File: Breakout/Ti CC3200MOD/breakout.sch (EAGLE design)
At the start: 69 parts, among them Q1 16Mhz, U1 TPS63001DRCT, U11 XL, U12 TMP006, U2 MCP73871-2CCI/ML, U5 93LC46BT-I/OT

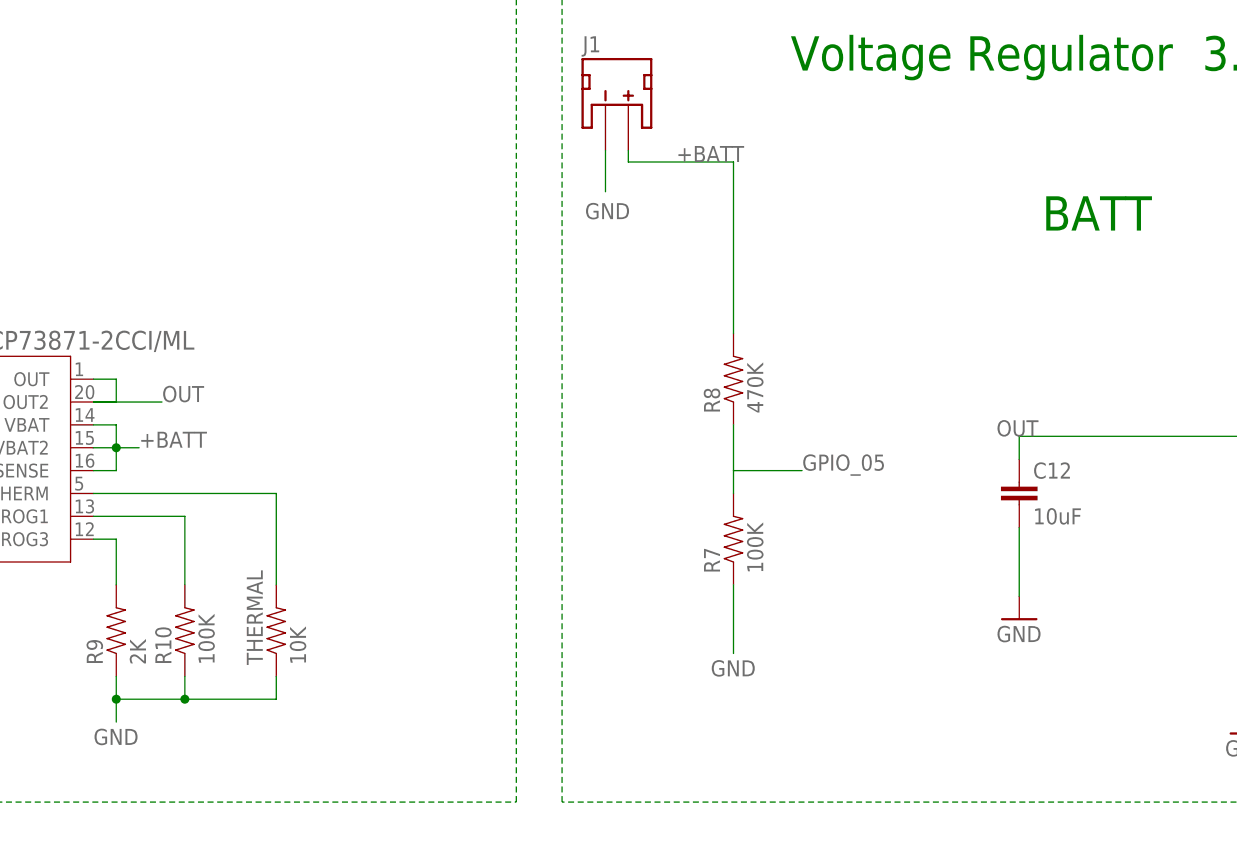
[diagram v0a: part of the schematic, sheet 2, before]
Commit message: Add Power Jumper
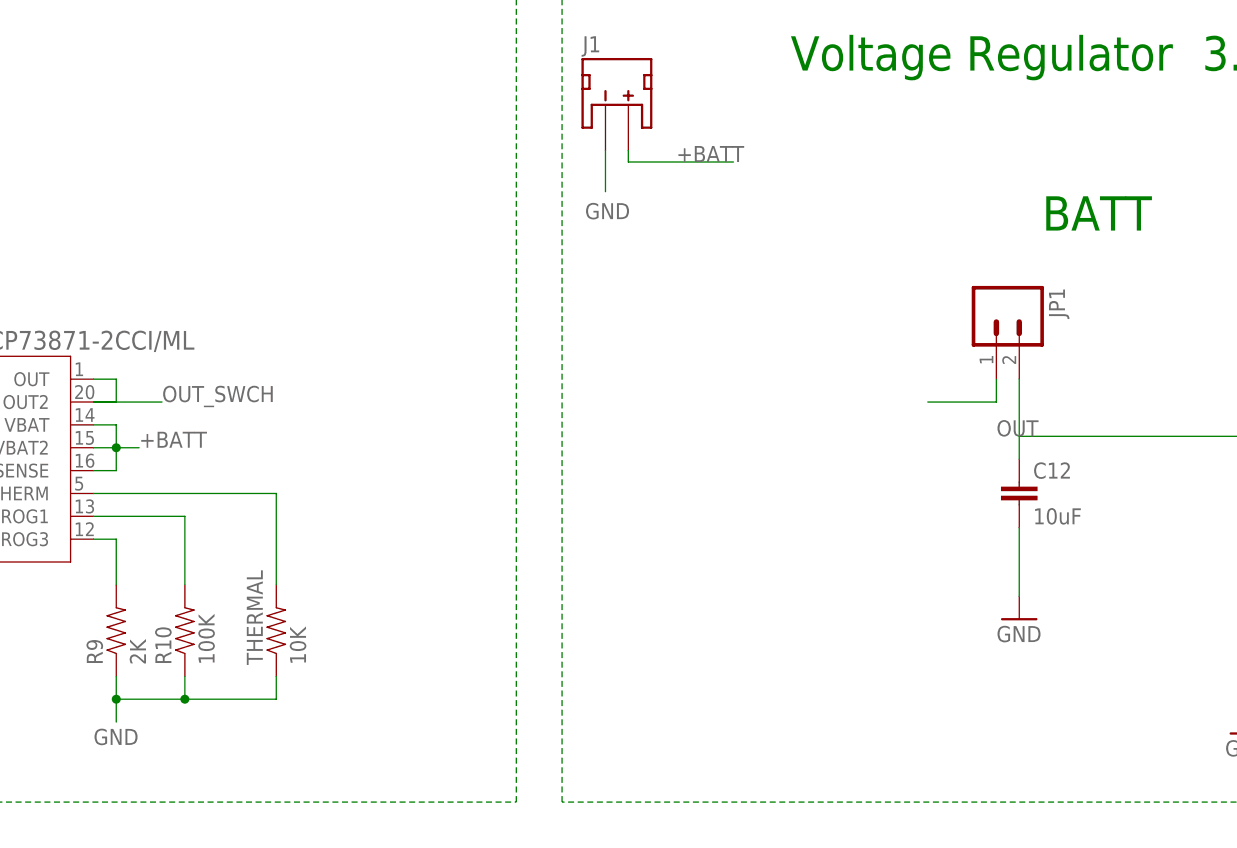
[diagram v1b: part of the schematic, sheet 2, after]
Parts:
- removed R7: 100K, SparkFun-Resistors:RESISTOR0603
- removed R8: 470K, SparkFun-Resistors:RESISTOR0603
- added JP1: (no value), DECADE-libraries:M02PTH
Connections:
- new net OUT_SWCH: JP1.1, U2.OUT, U2.OUT2
- net +BATT: no longer R8.2
- net GND: no longer R7.1
- net GPIO_05: no longer R7.2, R8.1
- net OUT: now also JP1.2; no longer U2.OUT, U2.OUT2
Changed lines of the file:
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@@
 <setting verticaltext="up"/>
 </settings>
-<grid distance="0.1" unitdist="inch" unit="inch" style="lines" multiple="1" display="no" altdistance="0.01" altunitdist="inch" altunit="inch"/>
+<grid distance="0.05" unitdist="inch" unit="inch" style="lines" multiple="1" display="no" altdistance="0.01" altunitdist="inch" altunit="inch"/>
 <layers>
 <layer number="1" name="Top" color="4" fill="1" visible="no" active="no"/>
@@
 <part name="R3" library="SparkFun-Resistors" deviceset="RESISTOR" device="0603" value="2.7K"/>
 <part name="SOP2" library="pinhead" deviceset="PINHD-1X2" device=""/>
-<part name="R7" library="SparkFun-Resistors" deviceset="RESISTOR" device="0603" value="100K"/>
-<part name="R8" library="SparkFun-Resistors" deviceset="RESISTOR" device="0603" value="470K"/>
 <part name="U2" library="microchip-battery" deviceset="MCP73871" device="ML" technology="-2CCI/"/>
 <part name="R9" library="SparkFun-Passives" deviceset="RESISTOR" device="0603-RES" value="2K"/>
@@
 <part name="R37" library="SparkFun-Passives" deviceset="RESISTOR" device="0603-RES" value="0R"/>
 <part name="C7" library="SparkFun-Capacitors" deviceset="CAP" device="0402-CAP" value=".1uF"/>
+<part name="JP1" library="DECADE-libraries" deviceset="M02" device="PTH"/>
 </parts>
 <sheets>
@@
 <instance part="USB" gate="G$1" x="30.48" y="350.52" rot="R180"/>
 <instance part="J1" gate="G$1" x="199.136" y="495.3"/>
-<instance part="R7" gate="G$1" x="213.36" y="447.04" rot="R90"/>
-<instance part="R8" gate="G$1" x="213.36" y="464.82" rot="R90"/>
 <instance part="U2" gate="A" x="124.46" y="457.2"/>
 <instance part="R9" gate="G$1" x="144.78" y="436.88" rot="R90"/>
@@
 <instance part="R37" gate="G$1" x="532.13" y="342.9" rot="R180"/>
 <instance part="C7" gate="G$1" x="472.44" y="363.22" rot="R270"/>
+<instance part="JP1" gate="G$1" x="242.57" y="472.44" rot="R270"/>
 </instances>
 <busses>
@@
 <wire x1="199.136" y1="490.22" x2="199.136" y2="485.648" width="0.1524" layer="91"/>
 <label x="196.85" y="482.6" size="1.778" layer="95"/>
-</segment>
-<segment>
-<pinref part="R7" gate="G$1" pin="1"/>
-<wire x1="213.36" y1="441.96" x2="213.36" y2="434.34" width="0.1524" layer="91"/>
-<label x="210.82" y="431.8" size="1.778" layer="95"/>
 </segment>
 <segment>
@@
 <wire x1="201.676" y1="488.95" x2="201.676" y2="490.22" width="0.1524" layer="91"/>
 <wire x1="201.676" y1="488.95" x2="213.36" y2="488.95" width="0.1524" layer="91"/>
-<pinref part="R8" gate="G$1" pin="2"/>
-<wire x1="213.36" y1="469.9" x2="213.36" y2="488.95" width="0.1524" layer="91"/>
 <label x="207.01" y="488.95" size="1.778" layer="95"/>
 </segment>
@@
 <wire x1="21.59" y1="417.83" x2="189.23" y2="417.83" width="0.1524" layer="91" style="longdash"/>
 <wire x1="189.23" y1="417.83" x2="189.23" y2="514.35" width="0.1524" layer="91" style="longdash"/>
-</segment>
-</net>
-<net name="GPIO_05" class="0">
-<segment>
-<pinref part="R8" gate="G$1" pin="1"/>
-<pinref part="R7" gate="G$1" pin="2"/>
-<wire x1="213.36" y1="459.74" x2="213.36" y2="454.66" width="0.1524" layer="91"/>
-<wire x1="213.36" y1="454.66" x2="213.36" y2="452.12" width="0.1524" layer="91"/>
-<wire x1="213.36" y1="454.66" x2="220.98" y2="454.66" width="0.1524" layer="91"/>
-<label x="220.98" y="454.66" size="1.778" layer="95"/>
 </segment>
 </net>
@@
 <wire x1="270.51" y1="450.85" x2="270.51" y2="453.39" width="0.1524" layer="91"/>
 <junction x="270.51" y="453.39"/>
-</segment>
-<segment>
-<pinref part="U2" gate="A" pin="OUT"/>
-<wire x1="142.24" y1="464.82" x2="144.78" y2="464.82" width="0.1524" layer="91"/>
-<wire x1="144.78" y1="464.82" x2="144.78" y2="462.28" width="0.1524" layer="91"/>
-<pinref part="U2" gate="A" pin="OUT2"/>
-<wire x1="144.78" y1="462.28" x2="142.24" y2="462.28" width="0.1524" layer="91"/>
-<wire x1="142.24" y1="462.28" x2="149.86" y2="462.28" width="0.1524" layer="91"/>
-<label x="149.86" y="462.28" size="1.778" layer="95"/>
+<pinref part="JP1" gate="G$1" pin="2"/>
+<wire x1="245.11" y1="458.47" x2="245.11" y2="464.82" width="0.1524" layer="91"/>
 </segment>
 </net>
@@
 </segment>
 </net>
+<net name="OUT_SWCH" class="0">
+<segment>
+<pinref part="U2" gate="A" pin="OUT"/>
+<wire x1="142.24" y1="464.82" x2="144.78" y2="464.82" width="0.1524" layer="91"/>
+<wire x1="144.78" y1="464.82" x2="144.78" y2="462.28" width="0.1524" layer="91"/>
+<pinref part="U2" gate="A" pin="OUT2"/>
+<wire x1="144.78" y1="462.28" x2="142.24" y2="462.28" width="0.1524" layer="91"/>
+<wire x1="142.24" y1="462.28" x2="149.86" y2="462.28" width="0.1524" layer="91"/>
+<label x="149.86" y="462.28" size="1.778" layer="95"/>
+</segment>
+<segment>
+<pinref part="JP1" gate="G$1" pin="1"/>
+<wire x1="242.57" y1="464.82" x2="242.57" y2="462.28" width="0.1524" layer="91"/>
+<wire x1="242.57" y1="462.28" x2="234.95" y2="462.28" width="0.1524" layer="91"/>
+</segment>
+</net>

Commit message: Revert "Add Power Jumper"
This reverts commit 700f51e2ac70f058cb62d27b6654cd07e4fedc2f.
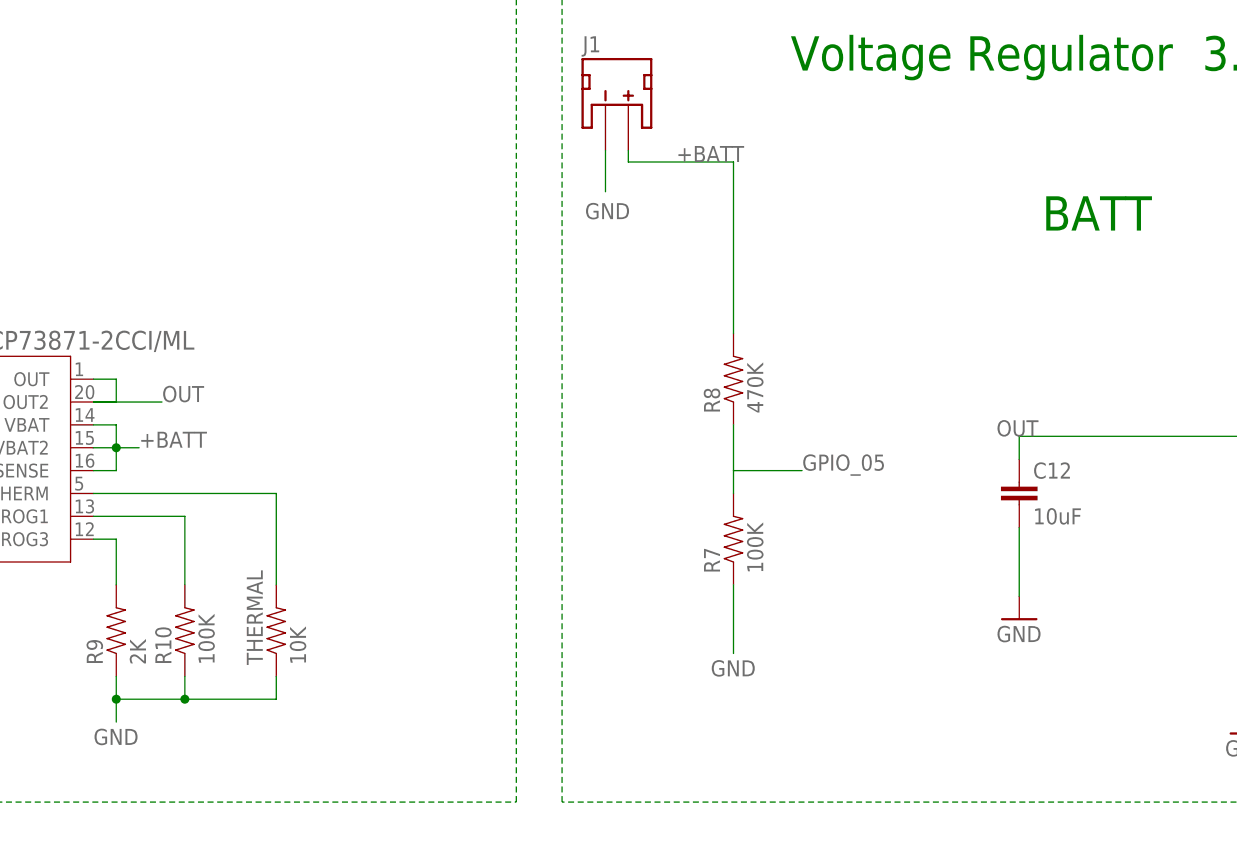
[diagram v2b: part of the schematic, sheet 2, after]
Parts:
- removed JP1: (no value), DECADE-libraries:M02PTH
- added R7: 100K, SparkFun-Resistors:RESISTOR0603
- added R8: 470K, SparkFun-Resistors:RESISTOR0603
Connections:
- removed net OUT_SWCH: JP1.1, U2.OUT, U2.OUT2
- net +BATT: now also R8.2
- net GND: now also R7.1
- net GPIO_05: now also R7.2, R8.1
- net OUT: now also U2.OUT, U2.OUT2; no longer JP1.2
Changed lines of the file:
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@@
 <setting verticaltext="up"/>
 </settings>
-<grid distance="0.05" unitdist="inch" unit="inch" style="lines" multiple="1" display="no" altdistance="0.01" altunitdist="inch" altunit="inch"/>
+<grid distance="0.1" unitdist="inch" unit="inch" style="lines" multiple="1" display="no" altdistance="0.01" altunitdist="inch" altunit="inch"/>
 <layers>
 <layer number="1" name="Top" color="4" fill="1" visible="no" active="no"/>
@@
 <part name="R3" library="SparkFun-Resistors" deviceset="RESISTOR" device="0603" value="2.7K"/>
 <part name="SOP2" library="pinhead" deviceset="PINHD-1X2" device=""/>
+<part name="R7" library="SparkFun-Resistors" deviceset="RESISTOR" device="0603" value="100K"/>
+<part name="R8" library="SparkFun-Resistors" deviceset="RESISTOR" device="0603" value="470K"/>
 <part name="U2" library="microchip-battery" deviceset="MCP73871" device="ML" technology="-2CCI/"/>
 <part name="R9" library="SparkFun-Passives" deviceset="RESISTOR" device="0603-RES" value="2K"/>
@@
 <part name="R37" library="SparkFun-Passives" deviceset="RESISTOR" device="0603-RES" value="0R"/>
 <part name="C7" library="SparkFun-Capacitors" deviceset="CAP" device="0402-CAP" value=".1uF"/>
-<part name="JP1" library="DECADE-libraries" deviceset="M02" device="PTH"/>
 </parts>
 <sheets>
@@
 <instance part="USB" gate="G$1" x="30.48" y="350.52" rot="R180"/>
 <instance part="J1" gate="G$1" x="199.136" y="495.3"/>
+<instance part="R7" gate="G$1" x="213.36" y="447.04" rot="R90"/>
+<instance part="R8" gate="G$1" x="213.36" y="464.82" rot="R90"/>
 <instance part="U2" gate="A" x="124.46" y="457.2"/>
 <instance part="R9" gate="G$1" x="144.78" y="436.88" rot="R90"/>
@@
 <instance part="R37" gate="G$1" x="532.13" y="342.9" rot="R180"/>
 <instance part="C7" gate="G$1" x="472.44" y="363.22" rot="R270"/>
-<instance part="JP1" gate="G$1" x="242.57" y="472.44" rot="R270"/>
 </instances>
 <busses>
@@
 <wire x1="199.136" y1="490.22" x2="199.136" y2="485.648" width="0.1524" layer="91"/>
 <label x="196.85" y="482.6" size="1.778" layer="95"/>
+</segment>
+<segment>
+<pinref part="R7" gate="G$1" pin="1"/>
+<wire x1="213.36" y1="441.96" x2="213.36" y2="434.34" width="0.1524" layer="91"/>
+<label x="210.82" y="431.8" size="1.778" layer="95"/>
 </segment>
 <segment>
@@
 <wire x1="201.676" y1="488.95" x2="201.676" y2="490.22" width="0.1524" layer="91"/>
 <wire x1="201.676" y1="488.95" x2="213.36" y2="488.95" width="0.1524" layer="91"/>
+<pinref part="R8" gate="G$1" pin="2"/>
+<wire x1="213.36" y1="469.9" x2="213.36" y2="488.95" width="0.1524" layer="91"/>
 <label x="207.01" y="488.95" size="1.778" layer="95"/>
 </segment>
@@
 <wire x1="21.59" y1="417.83" x2="189.23" y2="417.83" width="0.1524" layer="91" style="longdash"/>
 <wire x1="189.23" y1="417.83" x2="189.23" y2="514.35" width="0.1524" layer="91" style="longdash"/>
+</segment>
+</net>
+<net name="GPIO_05" class="0">
+<segment>
+<pinref part="R8" gate="G$1" pin="1"/>
+<pinref part="R7" gate="G$1" pin="2"/>
+<wire x1="213.36" y1="459.74" x2="213.36" y2="454.66" width="0.1524" layer="91"/>
+<wire x1="213.36" y1="454.66" x2="213.36" y2="452.12" width="0.1524" layer="91"/>
+<wire x1="213.36" y1="454.66" x2="220.98" y2="454.66" width="0.1524" layer="91"/>
+<label x="220.98" y="454.66" size="1.778" layer="95"/>
 </segment>
 </net>
@@
 <wire x1="270.51" y1="450.85" x2="270.51" y2="453.39" width="0.1524" layer="91"/>
 <junction x="270.51" y="453.39"/>
-<pinref part="JP1" gate="G$1" pin="2"/>
-<wire x1="245.11" y1="458.47" x2="245.11" y2="464.82" width="0.1524" layer="91"/>
+</segment>
+<segment>
+<pinref part="U2" gate="A" pin="OUT"/>
+<wire x1="142.24" y1="464.82" x2="144.78" y2="464.82" width="0.1524" layer="91"/>
+<wire x1="144.78" y1="464.82" x2="144.78" y2="462.28" width="0.1524" layer="91"/>
+<pinref part="U2" gate="A" pin="OUT2"/>
+<wire x1="144.78" y1="462.28" x2="142.24" y2="462.28" width="0.1524" layer="91"/>
+<wire x1="142.24" y1="462.28" x2="149.86" y2="462.28" width="0.1524" layer="91"/>
+<label x="149.86" y="462.28" size="1.778" layer="95"/>
 </segment>
 </net>
@@
 </segment>
 </net>
-<net name="OUT_SWCH" class="0">
-<segment>
-<pinref part="U2" gate="A" pin="OUT"/>
-<wire x1="142.24" y1="464.82" x2="144.78" y2="464.82" width="0.1524" layer="91"/>
-<wire x1="144.78" y1="464.82" x2="144.78" y2="462.28" width="0.1524" layer="91"/>
-<pinref part="U2" gate="A" pin="OUT2"/>
-<wire x1="144.78" y1="462.28" x2="142.24" y2="462.28" width="0.1524" layer="91"/>
-<wire x1="142.24" y1="462.28" x2="149.86" y2="462.28" width="0.1524" layer="91"/>
-<label x="149.86" y="462.28" size="1.778" layer="95"/>
-</segment>
-<segment>
-<pinref part="JP1" gate="G$1" pin="1"/>
-<wire x1="242.57" y1="464.82" x2="242.57" y2="462.28" width="0.1524" layer="91"/>
-<wire x1="242.57" y1="462.28" x2="234.95" y2="462.28" width="0.1524" layer="91"/>
-</segment>
-</net>
